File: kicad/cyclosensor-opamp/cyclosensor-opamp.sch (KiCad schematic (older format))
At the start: 12 parts, among them J1 RJ14, U1 LM358

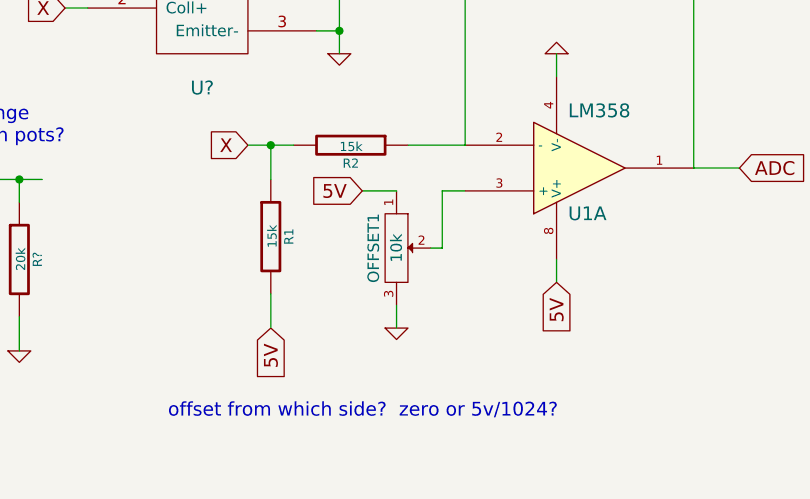
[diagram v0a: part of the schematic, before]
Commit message: tweak a few things
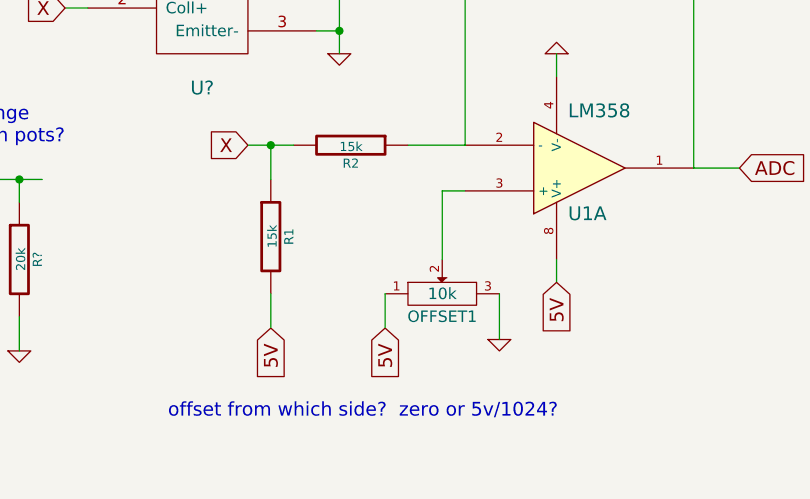
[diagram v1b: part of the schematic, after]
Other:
- moved on the sheet: OFFSET1
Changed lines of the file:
@@
 Sheet 1 1
 Title ""
-Date "13 apr 2014"
+Date "16 apr 2014"
 Rev ""
 Comp ""
@@
 L POT OFFSET1
 U 1 1 533BA12C
-P 4200 4800
-F 0 "OFFSET1" H 4200 4700 50  0000 C CNN
-F 1 "10k" H 4200 4800 50  0000 C CNN
-F 2 "~" H 4200 4800 60  0000 C CNN
-F 3 "~" H 4200 4800 60  0000 C CNN
-	1    4200 4800
-	0    1    1    0
-$EndComp
-Text GLabel 4050 4550 0    60   Input ~ 0
+P 4400 5000
+F 0 "OFFSET1" H 4400 4900 50  0000 C CNN
+F 1 "10k" H 4400 5000 50  0000 C CNN
+F 2 "~" H 4400 5000 60  0000 C CNN
+F 3 "~" H 4400 5000 60  0000 C CNN
+	1    4400 5000
+	1    0    0    -1
+$EndComp
+Text GLabel 4150 5150 3    60   Input ~ 0
 5V
 NoConn ~ 7100 3500
@@
 L GND #PWR?
 U 1 1 5349C88D
-P 4200 5150
-F 0 "#PWR?" H 4200 5150 30  0001 C CNN
-F 1 "GND" H 4200 5080 30  0001 C CNN
-F 2 "" H 4200 5150 60  0000 C CNN
-F 3 "" H 4200 5150 60  0000 C CNN
-	1    4200 5150
-	1    0    0    -1
-$EndComp
-Wire Wire Line
-	4350 4800 4400 4800
-Wire Wire Line
-	4400 4800 4400 4550
+P 4650 5200
+F 0 "#PWR?" H 4650 5200 30  0001 C CNN
+F 1 "GND" H 4650 5130 30  0001 C CNN
+F 2 "" H 4650 5200 60  0000 C CNN
+F 3 "" H 4650 5200 60  0000 C CNN
+	1    4650 5200
+	1    0    0    -1
+$EndComp
+Wire Wire Line
+	4400 4550 4400 4850
 Wire Wire Line
 	4400 4550 4500 4550
 Wire Wire Line
-	4050 4550 4200 4550
-Wire Wire Line
-	4200 5150 4200 5050
+	4150 5150 4150 5000
 Text Notes 1850 4350 0    60   ~ 0
 not used - change\nback to save on pots?
+Wire Wire Line
+	4650 5000 4650 5200
 $EndSCHEMATC
